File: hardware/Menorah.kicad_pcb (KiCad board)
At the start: 2 copper layers, 111.8 x 130.3 mm, 21 parts, among them SW1 SW_Push, U1 ATtiny85-20PU

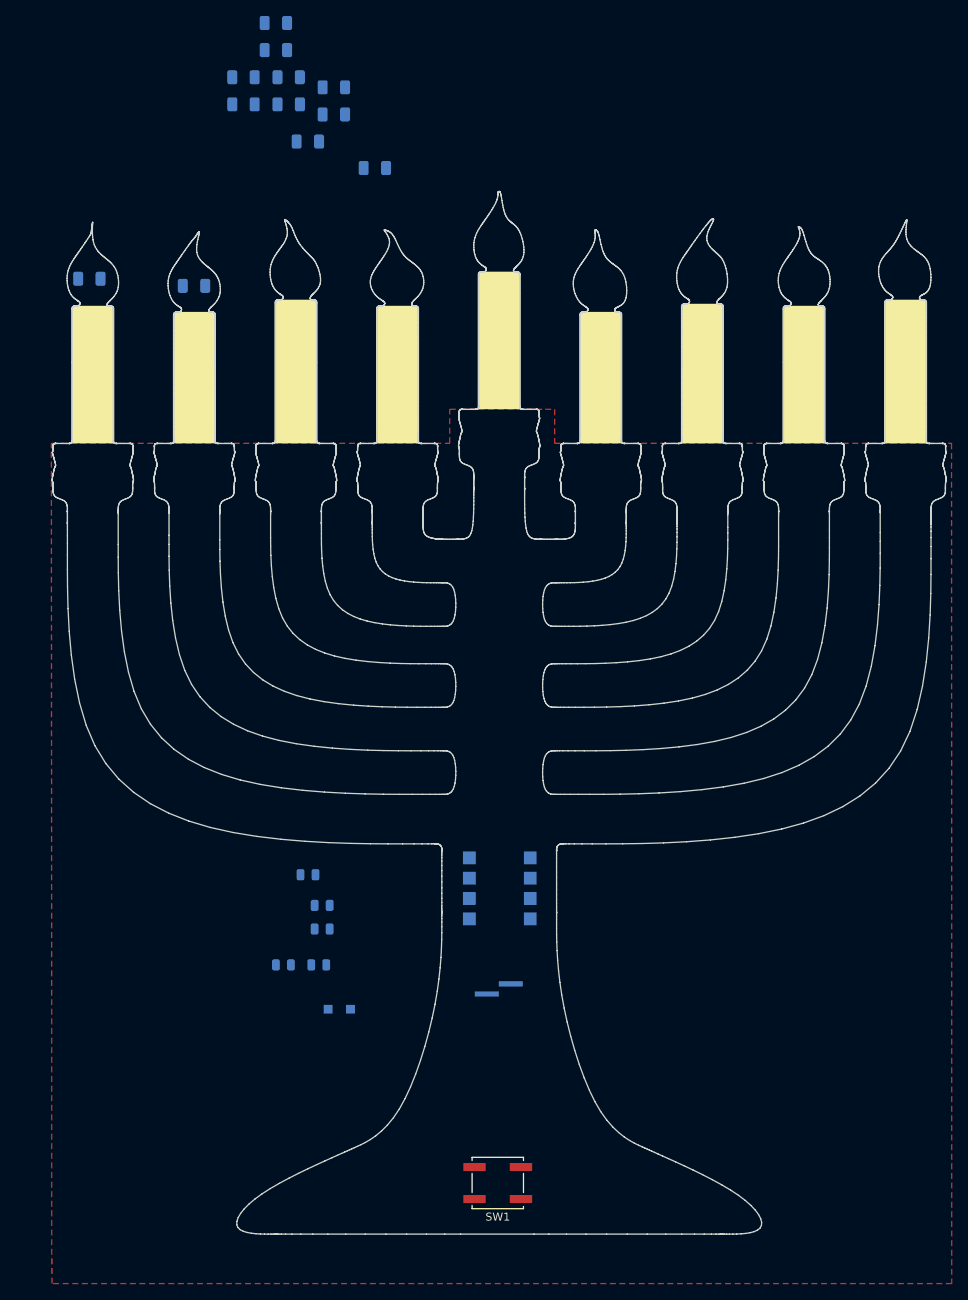
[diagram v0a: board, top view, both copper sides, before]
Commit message: lotsa stuff
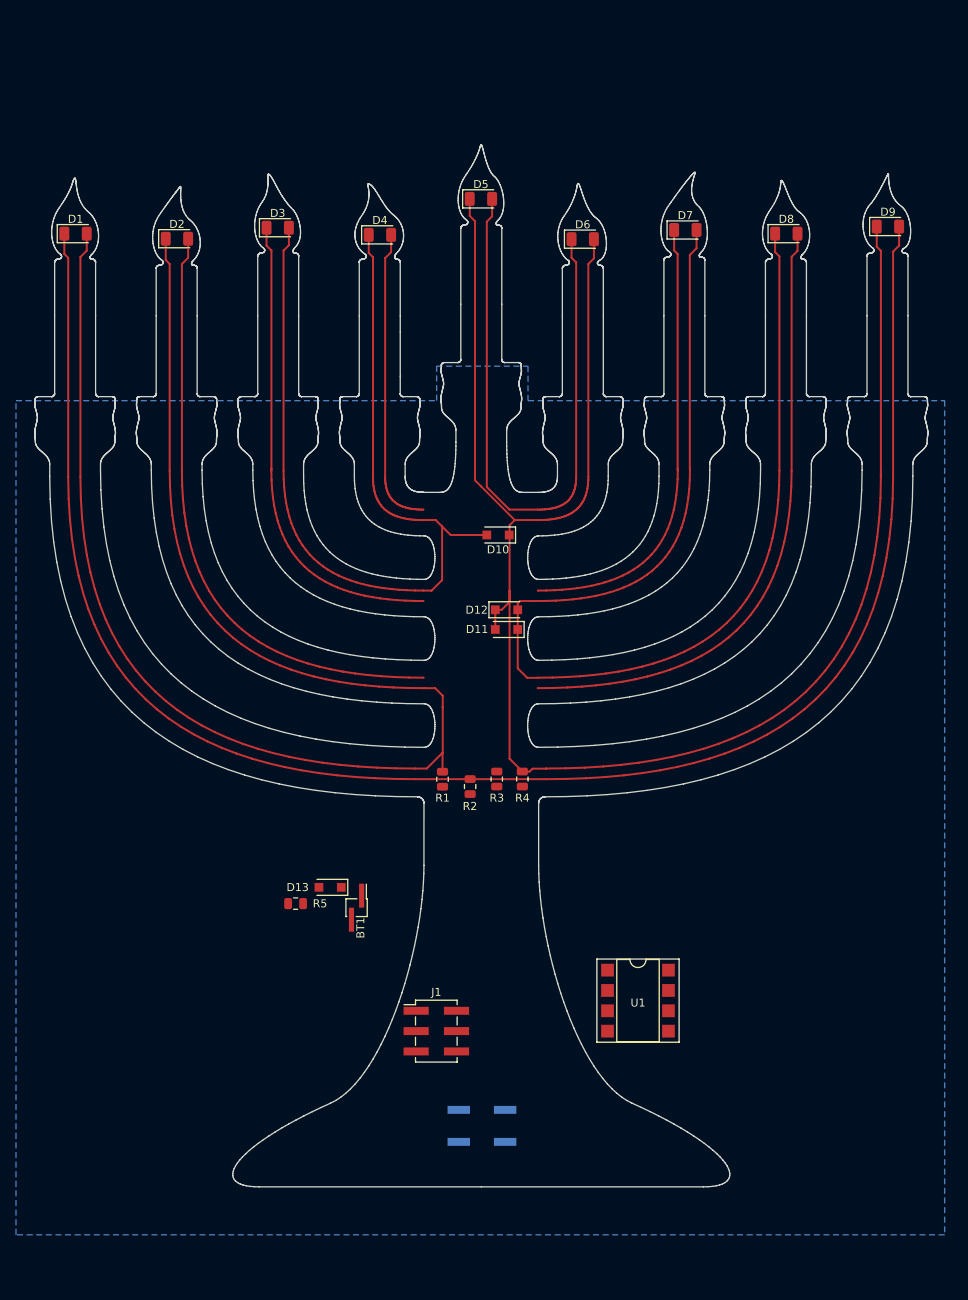
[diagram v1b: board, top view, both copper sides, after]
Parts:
- added G***: LOGO, menorah:menorah_mask, F.Cu at (142.0, 103.9)
- added G***: LOGO, menorah:menorah_traces, F.Cu at (141.4, 83.9)
- added J1: Conn_02x03_Odd_Even, Connector_PinHeader_2.54mm:PinHeader_2x03_P2.54mm_Vertical_SMD, F.Cu at (136.3, 132.3)
- BT1, D1, D13, D2, D3, D4, D5, D6, D7, D8, D9, R1, R2, R3, R4, R5, U1: moved to F.Cu
- D10, D11, D12: value LED -> 1N4004; footprint LED_SMD:LED_1206_3216Metric -> Diode_SMD:D_SOD-123F; moved to F.Cu
- SW1: moved to B.Cu
- moved D11 81.1 mm to (145.1, 82.1), turned to 180 degrees
- moved D9 70.7 mm to (192.8, 31.7)
- moved D12 68.8 mm to (145.1, 79.6)
- moved D7 53.1 mm to (167.5, 32.1)
- moved D8 52.1 mm to (180.1, 32.6)
- moved D5 50.0 mm to (141.9, 28.2)
- moved D10 49.1 mm to (144.0, 70.3), turned to 180 degrees
- moved D6 45.0 mm to (154.6, 33.3)
- moved R2 32.3 mm to (140.6, 101.7), turned to 270 degrees
- moved R4 29.3 mm to (147.1, 100.8), turned to 270 degrees
- moved R3 26.9 mm to (143.9, 100.8), turned to 270 degrees
- moved D1 26.5 mm to (91.2, 32.6)
- moved R1 24.0 mm to (137.1, 100.8), turned to 270 degrees
- moved U1 22.3 mm to (161.5, 128.5)
- moved D2 21.8 mm to (103.9, 33.2)
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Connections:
- net Net-(D13-Pad2) renamed VCC
- net Net-(R1-Pad2) renamed MISO
- net Net-(R2-Pad2) renamed SCK
- net Net-(R5-Pad1) renamed MOSI
- D10 pad 2: Net-(D1-Pad2) -> Net-(D1-Pad1)
- D11 pad 1: Net-(D1-Pad1) -> Net-(D1-Pad2)
- D12 pad 1: Net-(D1-Pad2) -> Net-(D10-Pad1)
- D12 pad 2: Net-(D10-Pad1) -> Net-(D1-Pad2)
- D6 pad 2: Net-(D1-Pad2) -> Net-(D10-Pad1)
- D7 pad 2: Net-(D10-Pad1) -> Net-(D1-Pad2)
- U1 pad 1: Net-(U1-Pad1) -> RST
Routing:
- net Net-(D3-Pad1): track 0.00 -> 195.2 mm
- net Net-(D1-Pad1): track 0.00 -> 188.0 mm
- net Net-(D1-Pad2): track 0.00 -> 150.7 mm
- net Net-(D10-Pad1): track 0.00 -> 149.0 mm
- added copper zone on B.Cu, net GND
- removed copper zone on F.Cu, net GND
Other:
- board size 111.8 x 130.3 mm -> 111.6 x 130.3 mm
